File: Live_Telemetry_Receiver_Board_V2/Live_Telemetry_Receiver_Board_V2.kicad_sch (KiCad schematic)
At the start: 4 parts, among them CN1 NUCLEO-L432KC, U1 XBP9B-DPST-001

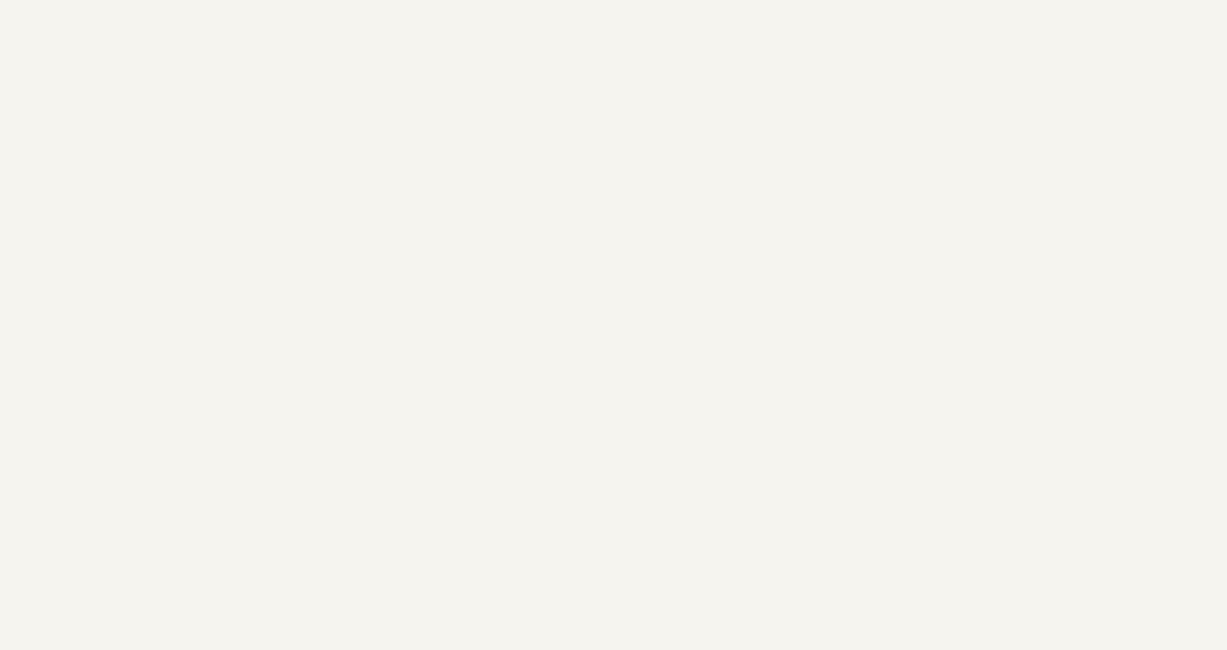
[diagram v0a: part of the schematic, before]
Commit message: save
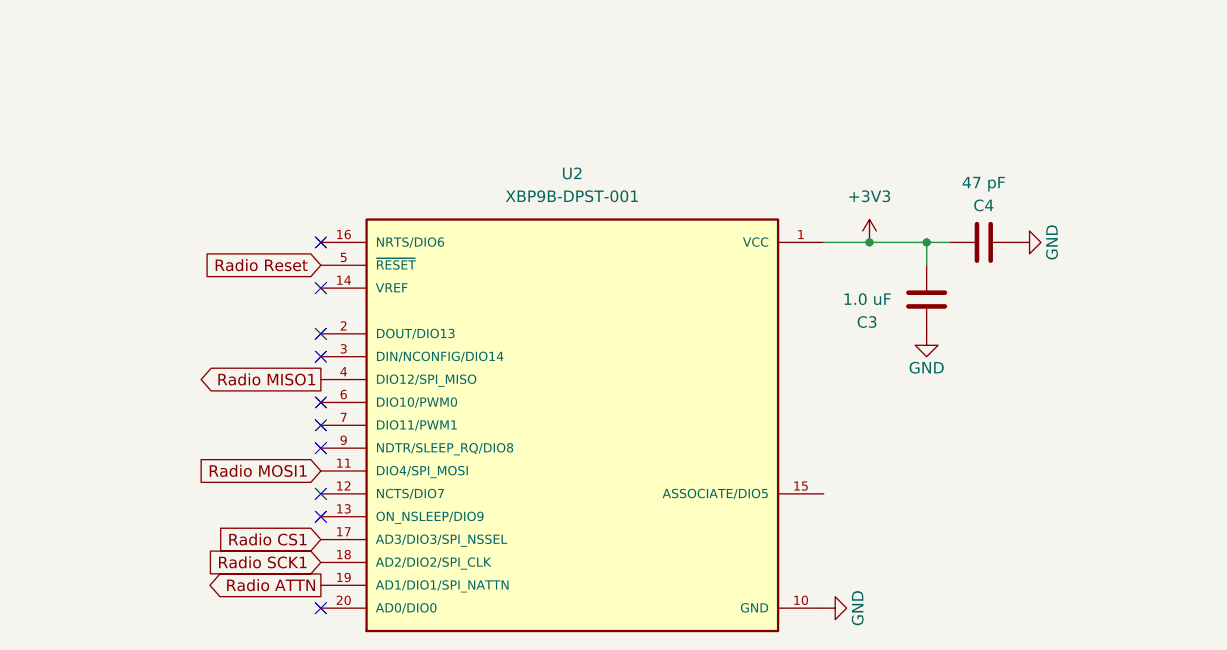
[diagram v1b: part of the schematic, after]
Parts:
- added C3: 1.0 uF, Capacitor_SMD:C_0805_2012Metric_Pad1.18x1.45mm_HandSolder, symbol Device:C
- added C4: 47 pF, Capacitor_SMD:C_0805_2012Metric_Pad1.18x1.45mm_HandSolder, symbol Device:C
- added U2: XBP9B-DPST-001, FS_3_Global_Footprint_Library:XBP9B-DPST-001, symbol FS_3_Global_Symbol_Library:XBP9B-DPST-001
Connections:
- net +3V3: now also C3.1, C4.1, U2.1 (VCC)
- net GND: now also C3.2, C4.2, U2.10 (GND)
- new net Radio ATTN: U2.19 (AD1/DIO1/SPI_NATTN)
- new net Radio CS1: U2.17 (AD3/DIO3/SPI_NSSEL)
- new net Radio MISO1: U2.4 (DIO12/SPI_MISO)
- new net Radio MOSI1: U2.11 (DIO4/SPI_MOSI)
- new net Radio Reset: U2.5 (~{RESET})
- new net Radio SCK1: U2.18 (AD2/DIO2/SPI_CLK)
- no-connect marks 0 -> 10

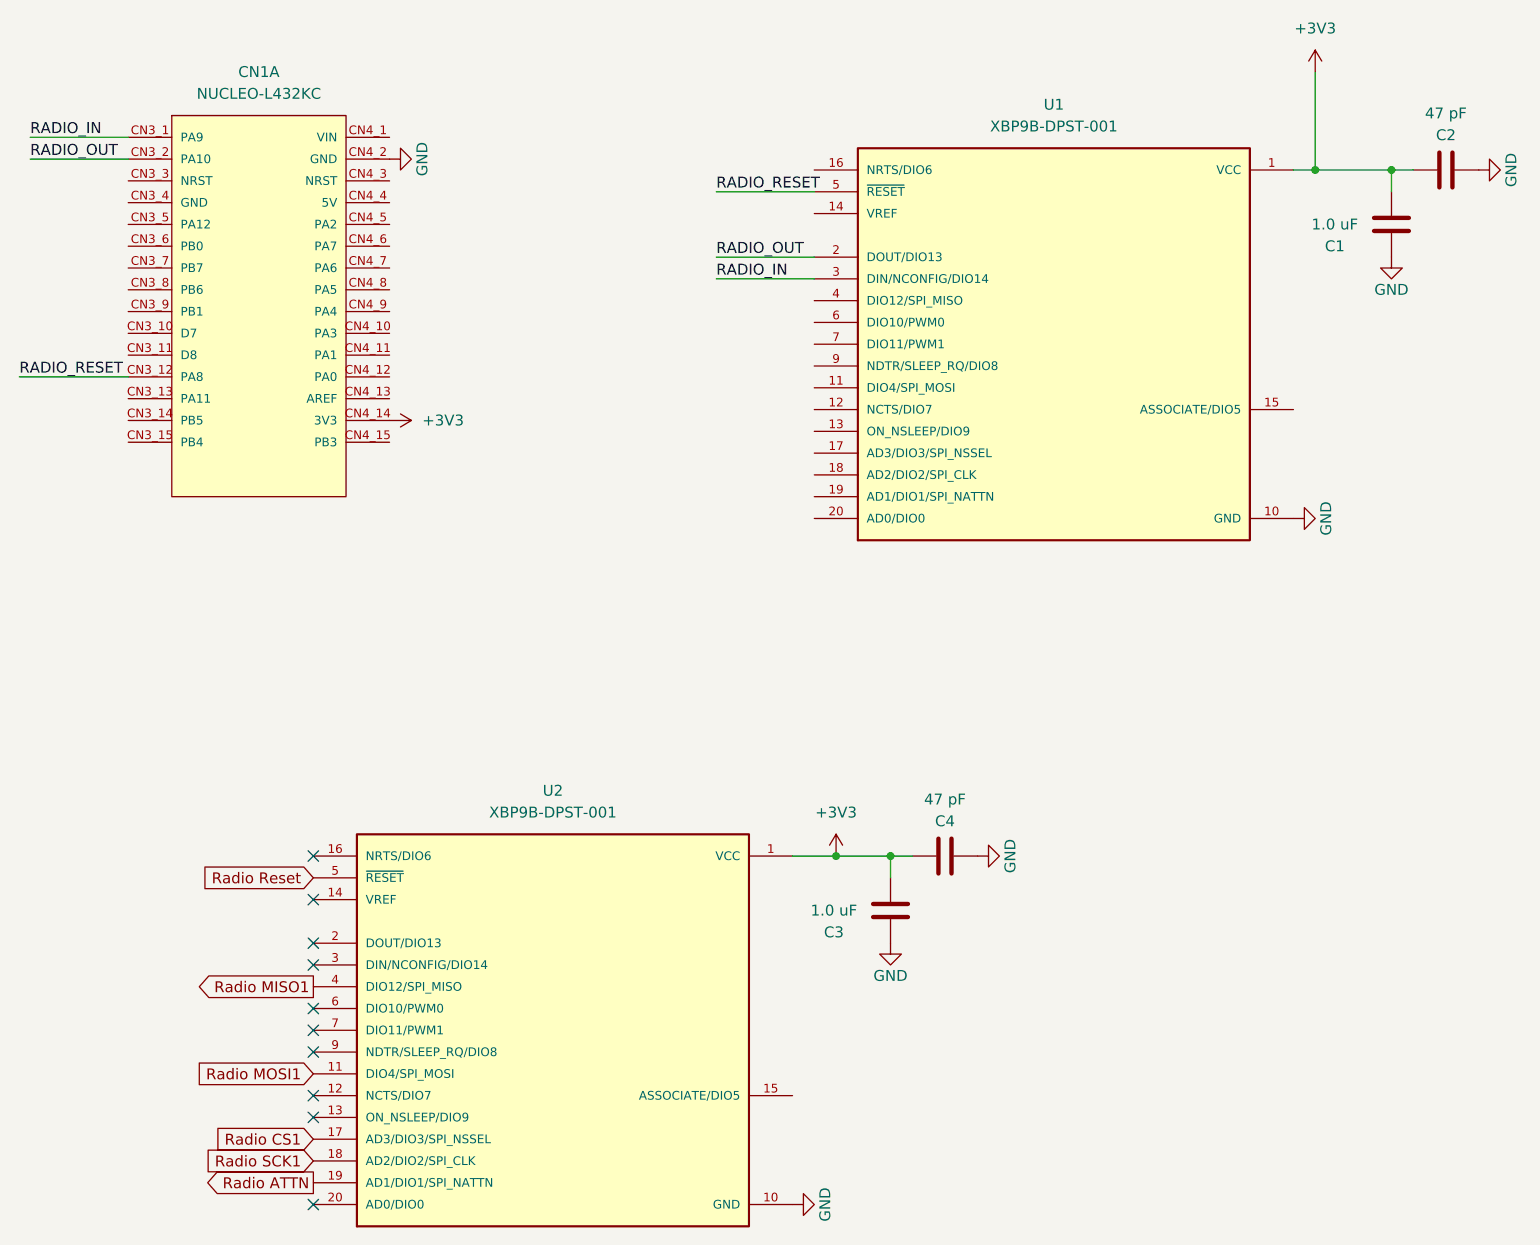
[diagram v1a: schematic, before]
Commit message: update LT Receiver V2 Schem (PCB not done)
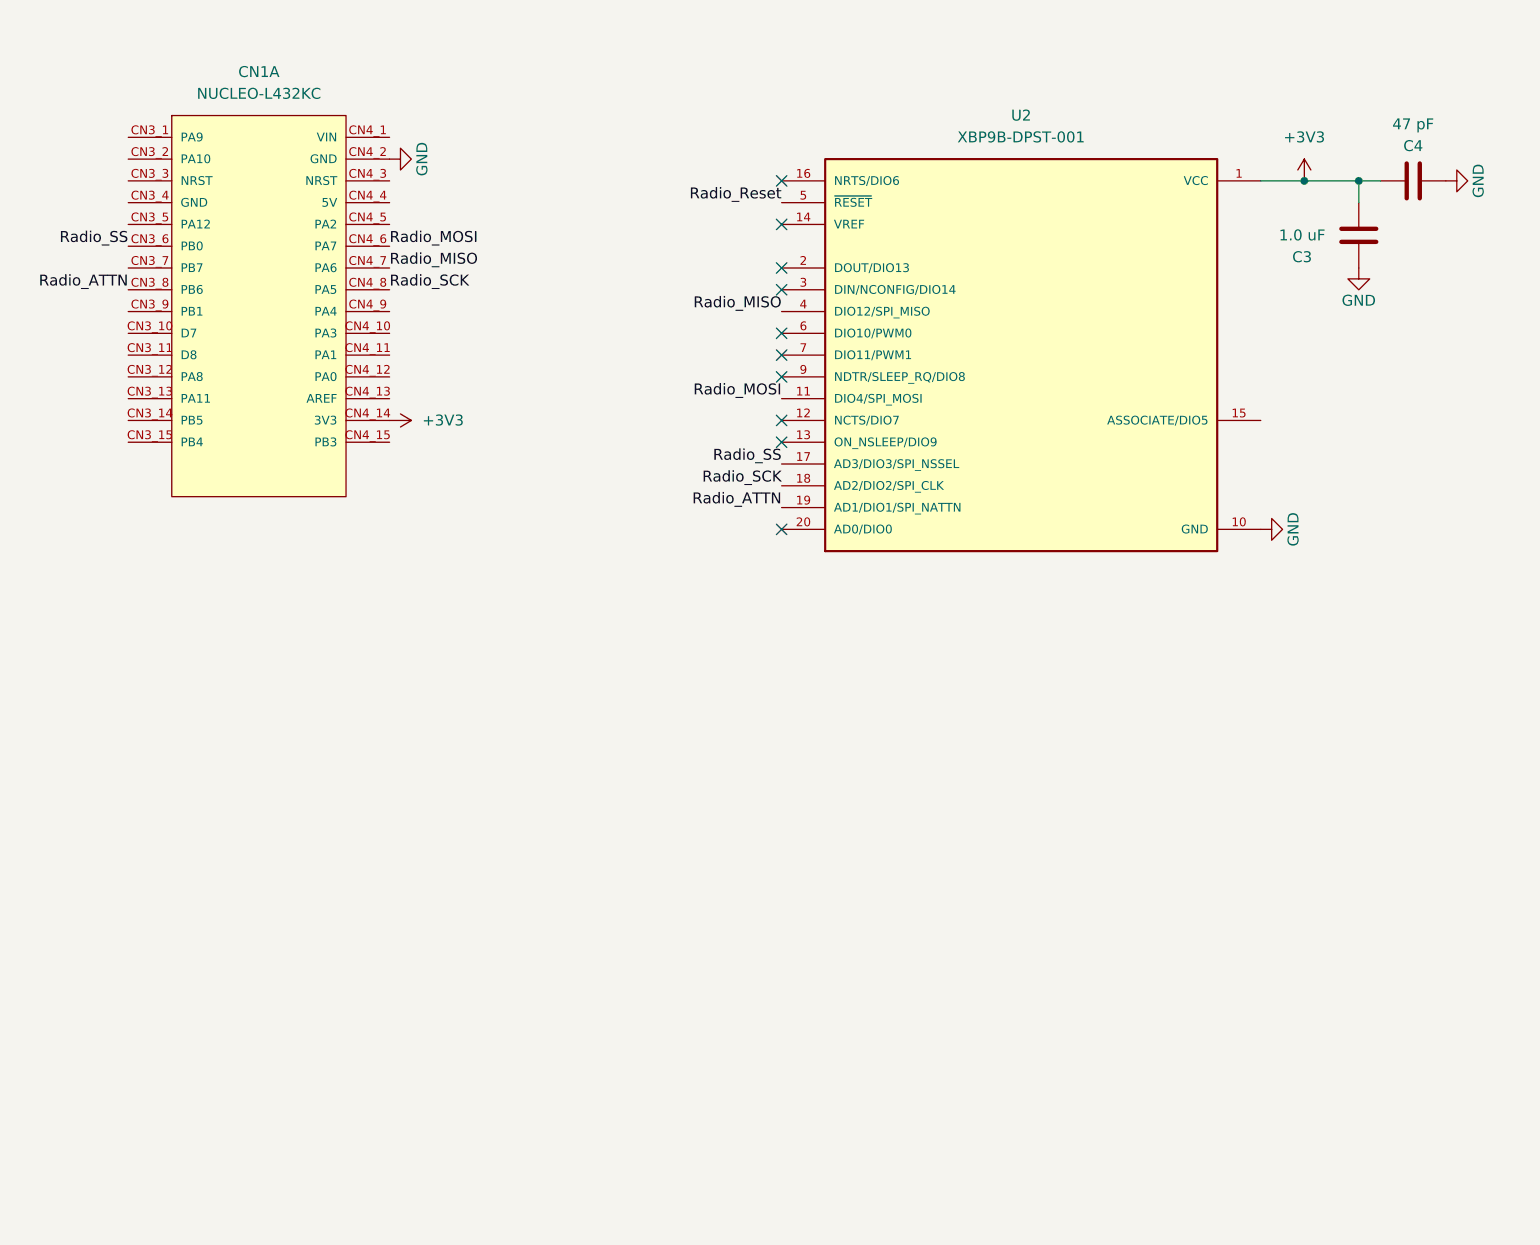
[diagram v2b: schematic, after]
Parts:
- removed C1: 1.0 uF, Capacitor_SMD:C_0805_2012Metric_Pad1.18x1.45mm_HandSolder, symbol Device:C
- removed C2: 47 pF, Capacitor_SMD:C_0805_2012Metric_Pad1.18x1.45mm_HandSolder, symbol Device:C
- removed U1: XBP9B-DPST-001, FS_3_Global_Footprint_Library:XBP9B-DPST-001, symbol FS_3_Global_Symbol_Library:XBP9B-DPST-001
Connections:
- net Radio ATTN is gone; now on net Radio_ATTN: U2.19 (AD1/DIO1/SPI_NATTN)
- net Radio CS1 is gone; now on net Radio_SS: U2.17 (AD3/DIO3/SPI_NSSEL)
- net Radio MISO1 is gone; now on net Radio_MISO: U2.4 (DIO12/SPI_MISO)
- net Radio MOSI1 is gone; now on net Radio_MOSI: U2.11 (DIO4/SPI_MOSI)
- net Radio SCK1 is gone; now on net Radio_SCK: U2.18 (AD2/DIO2/SPI_CLK)
- net Radio_SS: now reaches CN1.CN3_6 (PB0)
- net Radio_ATTN: now reaches CN1.CN3_8 (PB6)
- net Radio_MOSI: now reaches CN1.CN4_6 (PA7)
- net Radio_MISO: now reaches CN1.CN4_7 (PA6)
- net Radio_SCK: now reaches CN1.CN4_8 (PA5)
- net RADIO_IN: no longer names the net of CN1.CN3_1 (PA9)
- net RADIO_OUT: no longer names the net of CN1.CN3_2 (PA10)
- net RADIO_RESET: no longer names the net of CN1.CN3_12 (PA8)
- net Radio Reset renamed Radio_Reset
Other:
- moved on the sheet: C3, C4, U2
